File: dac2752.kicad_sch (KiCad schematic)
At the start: 24 parts, among them U30 LTC2752B, U301 OPA2197D, U31 OPA2189DGK, U32 OPA2388DGK, U34 OPA2388DGK

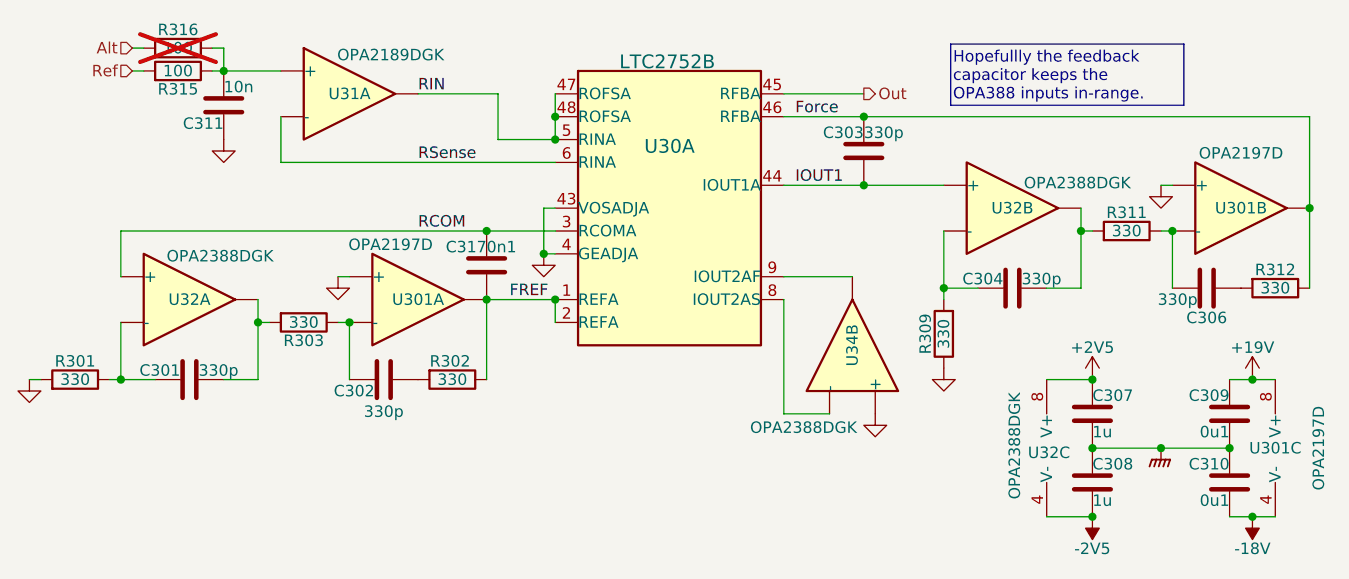
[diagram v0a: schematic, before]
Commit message: Progress checkin.  About to redo FDA feedback again.
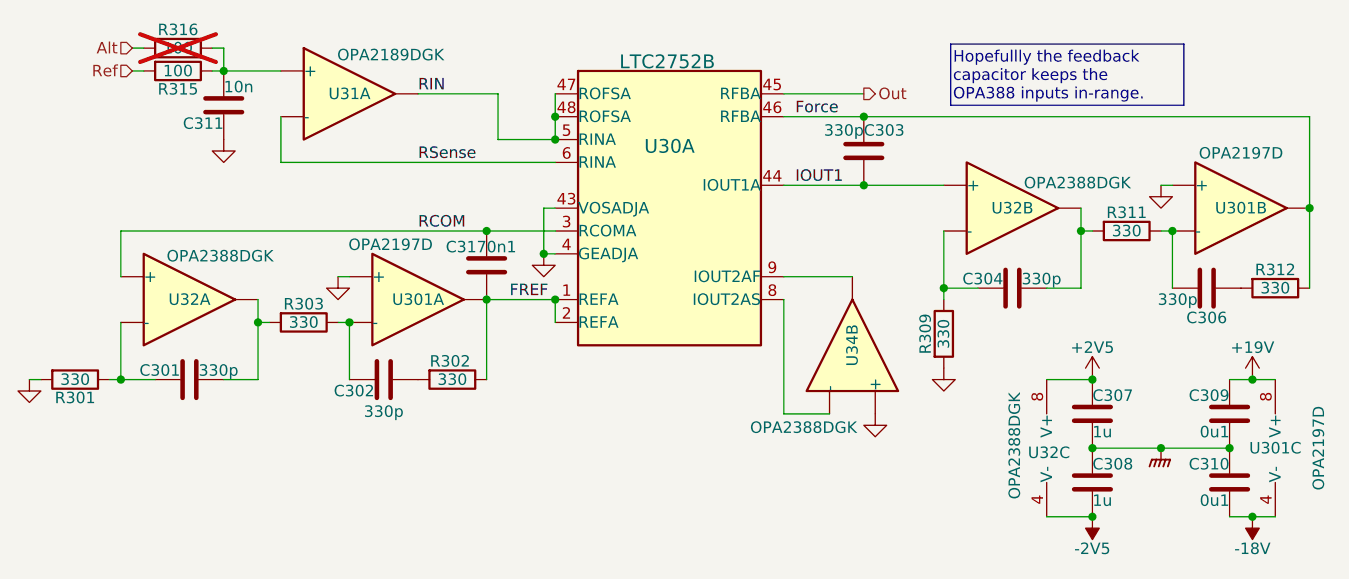
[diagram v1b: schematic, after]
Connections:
- net Alt: now also R316.1; no longer R316.2
- net Force: now also C303.1; no longer C303.2
- net GND: now also R309.2; no longer R309.1
- net IOUT1: now also C303.2; no longer C303.1
- net at C304.2, U32.6 (-): now also R309.1; no longer R309.2
- net at C311.1, R315.1, U31.3 (+): now also R316.2; no longer R316.1
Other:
- moved on the sheet: C303, R309, R316
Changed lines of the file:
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@@
 	)
 	(junction
-		(at 170.18 118.11)
+		(at 144.78 81.28)
 		(diameter 0)
 		(color 0 0 0 0)
 	)
 	(junction
-		(at 110.49 81.28)
+		(at 170.18 118.11)
 		(diameter 0)
 		(color 0 0 0 0)
 	)
 	(junction
-		(at 153.67 100.33)
+		(at 110.49 81.28)
 		(diameter 0)
 		(color 0 0 0 0)
 	)
 	(junction
-		(at 102.87 101.6)
+		(at 153.67 100.33)
 		(diameter 0)
 		(color 0 0 0 0)
 	)
 	(junction
-		(at 144.78 81.28)
+		(at 102.87 101.6)
 		(diameter 0)
 		(color 0 0 0 0)
@@
 	)
 	(junction
-		(at 144.78 88.9)
-		(diameter 0)
-		(color 0 0 0 0)
-	)
-	(junction
 		(at 168.91 93.98)
 		(diameter 0)
@@
 	)
 	(junction
+		(at 144.78 88.9)
+		(diameter 0)
+		(color 0 0 0 0)
+	)
+	(junction
 		(at 73.66 76.2)
 		(diameter 0)
@@
 	(wire
 		(pts
-			(xy 144.78 81.28) (xy 194.31 81.28)
+			(xy 72.39 73.66) (xy 73.66 73.66)
 		)
 		(stroke
@@
 	(wire
 		(pts
-			(xy 72.39 73.66) (xy 73.66 73.66)
+			(xy 73.66 73.66) (xy 73.66 76.2)
 		)
 		(stroke
@@
 	(wire
 		(pts
-			(xy 73.66 73.66) (xy 73.66 76.2)
+			(xy 80.01 81.28) (xy 80.01 86.36)
 		)
 		(stroke
@@
 	(wire
 		(pts
-			(xy 80.01 81.28) (xy 80.01 86.36)
+			(xy 63.5 76.2) (xy 64.77 76.2)
 		)
 		(stroke
@@
 	(wire
 		(pts
-			(xy 63.5 76.2) (xy 64.77 76.2)
+			(xy 62.23 99.06) (xy 62.23 93.98)
 		)
 		(stroke
@@
 	(wire
 		(pts
-			(xy 62.23 99.06) (xy 62.23 93.98)
+			(xy 66.04 110.49) (xy 62.23 110.49)
 		)
 		(stroke
@@
 	(wire
 		(pts
-			(xy 66.04 110.49) (xy 62.23 110.49)
+			(xy 144.78 88.9) (xy 153.67 88.9)
 		)
 		(stroke
@@
 	(wire
 		(pts
+			(xy 144.78 81.28) (xy 194.31 81.28)
+		)
+		(stroke
+			(width 0)
+			(type default)
+		)
+	)
+	(wire
+		(pts
 			(xy 102.87 93.98) (xy 110.49 93.98)
 		)
@@
 	(wire
 		(pts
-			(xy 144.78 88.9) (xy 153.67 88.9)
-		)
-		(stroke
-			(width 0)
-			(type default)
-		)
-	)
-	(wire
-		(pts
 			(xy 102.87 101.6) (xy 102.87 110.49)
 		)
@@
 		(lib_id "Device:C")
 		(at 170.18 114.3 0)
-		(mirror y)
 		(unit 1)
 		(exclude_from_sim no)
@@
 					(size 1.27 1.27)
 				)
-				(justify right)
+				(justify left)
 			)
 		)
@@
 					(size 1.27 1.27)
 				)
-				(justify right top)
+				(justify left top)
 			)
 		)
 		(property "Footprint" "Capacitor_SMD:C_0402_1005Metric"
-			(at 169.2148 118.11 0)
+			(at 171.1452 118.11 0)
 			(effects
 				(font
@@
 		(dnp no)
 		(property "Reference" "R303"
-			(at 82.55 106.172 90)
+			(at 82.55 102.108 90)
 			(effects
 				(font
@@
 		(lib_id "Device:R")
 		(at 57.15 110.49 270)
-		(mirror x)
 		(unit 1)
 		(exclude_from_sim no)
@@
 		(dnp no)
 		(property "Reference" "R301"
-			(at 57.15 108.458 90)
+			(at 57.15 112.522 90)
 			(effects
 				(font
@@
 		)
 		(property "Footprint" "Resistor_SMD:R_0402_1005Metric"
-			(at 57.15 112.268 90)
+			(at 57.15 108.712 90)
 			(effects
 				(font
@@
 		(lib_id "Device:C")
 		(at 185.42 114.3 0)
-		(mirror y)
 		(unit 1)
 		(exclude_from_sim no)
@@
 					(size 1.27 1.27)
 				)
-				(justify left)
+				(justify right)
 			)
 		)
@@
 					(size 1.27 1.27)
 				)
-				(justify left top)
+				(justify right top)
 			)
 		)
 		(property "Footprint" "Capacitor_SMD:C_0402_1005Metric"
-			(at 184.4548 118.11 0)
+			(at 186.3852 118.11 0)
 			(effects
 				(font
@@
 		(lib_id "Device:C")
 		(at 69.85 110.49 270)
-		(mirror x)
 		(unit 1)
 		(exclude_from_sim no)
@@
 		)
 		(property "Footprint" "Capacitor_SMD:C_0603_1608Metric"
-			(at 66.04 109.5248 0)
+			(at 66.04 111.4552 0)
 			(effects
 				(font
@@
 	(symbol
 		(lib_id "Device:C")
-		(at 144.78 85.09 180)
+		(at 144.78 85.09 0)
 		(unit 1)
 		(exclude_from_sim no)
@@
 		(dnp no)
 		(property "Reference" "C303"
-			(at 144.78 83.058 0)
+			(at 144.78 82.804 0)
 			(effects
 				(font
@@
 		)
 		(property "Value" "330p"
-			(at 144.78 83.058 0)
+			(at 144.78 82.804 0)
 			(effects
 				(font
@@
 		)
 		(property "Footprint" "Capacitor_SMD:C_0603_1608Metric"
-			(at 143.8148 81.28 0)
+			(at 145.7452 88.9 0)
 			(effects
 				(font
@@
 	(symbol
 		(lib_id "Device:R")
-		(at 68.58 73.66 270)
-		(mirror x)
+		(at 68.58 73.66 90)
 		(unit 1)
 		(exclude_from_sim no)
@@
 		(lib_id "Device:C")
 		(at 170.18 121.92 0)
-		(mirror y)
 		(unit 1)
 		(exclude_from_sim no)
@@
 					(size 1.27 1.27)
 				)
-				(justify right)
+				(justify left)
 			)
 		)
@@
 					(size 1.27 1.27)
 				)
-				(justify right top)
+				(justify left top)
 			)
 		)
 		(property "Footprint" "Capacitor_SMD:C_0402_1005Metric"
-			(at 169.2148 125.73 0)
+			(at 171.1452 125.73 0)
 			(effects
 				(font
@@
 	(symbol
 		(lib_id "Device:R")
-		(at 153.67 105.41 180)
+		(at 153.67 105.41 0)
 		(unit 1)
 		(exclude_from_sim no)
@@
 		)
 		(property "Footprint" "Resistor_SMD:R_0402_1005Metric"
-			(at 155.448 105.41 90)
+			(at 151.892 105.41 90)
 			(effects
 				(font
@@
 		(lib_id "Device:R")
 		(at 173.99 93.98 270)
-		(mirror x)
 		(unit 1)
 		(exclude_from_sim no)
@@
 		)
 		(property "Footprint" "Resistor_SMD:R_0402_1005Metric"
-			(at 173.99 95.758 90)
+			(at 173.99 92.202 90)
 			(effects
 				(font
@@
 		(lib_id "Device:R")
 		(at 68.58 76.2 270)
-		(mirror x)
 		(unit 1)
 		(exclude_from_sim no)
@@
 		)
 		(property "Footprint" "Resistor_SMD:R_0603_1608Metric"
-			(at 68.58 77.978 90)
+			(at 68.58 74.422 90)
 			(effects
 				(font
@@
 		(lib_id "Device:C")
 		(at 161.29 100.33 270)
-		(mirror x)
 		(unit 1)
 		(exclude_from_sim no)
@@
 		)
 		(property "Footprint" "Capacitor_SMD:C_0603_1608Metric"
-			(at 157.48 99.3648 0)
+			(at 157.48 101.2952 0)
 			(effects
 				(font
@@
 		(lib_id "Device:C")
 		(at 185.42 121.92 0)
-		(mirror y)
 		(unit 1)
 		(exclude_from_sim no)
@@
 					(size 1.27 1.27)
 				)
-				(justify left)
+				(justify right)
 			)
 		)
@@
 					(size 1.27 1.27)
 				)
-				(justify left top)
+				(justify right top)
 			)
 		)
 		(property "Footprint" "Capacitor_SMD:C_0402_1005Metric"
-			(at 184.4548 125.73 0)
+			(at 186.3852 125.73 0)
 			(effects
 				(font
